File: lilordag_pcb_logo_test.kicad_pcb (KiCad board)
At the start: 2 copper layers, 98.1 x 100 mm, 178 parts, among them J1 USB4105-GF-A, J2 826629-7, J3 826629-7, Q1 BC846, Q2 BC846, Q3 MMBT3906, Q4 MMBT3906, Q5 BC846, Q6 BC846, Q7 SSM3J56MFV, Q8 SSM3J56MFV, SW1 PCM12SMTR, SW2 PCM12SMTR, SW3 SW_MEC_5G, SW4 PCM12SMTR, SW5 SW_MEC_5G, SW6 SW_MEC_5G, SW7 SW_MEC_5G, U1 ESP32-C3-MINI-1-N4, U2 WS2812B-B, U3 WS2812B-B, U4 WS2812B-B, U5 WS2812B-B

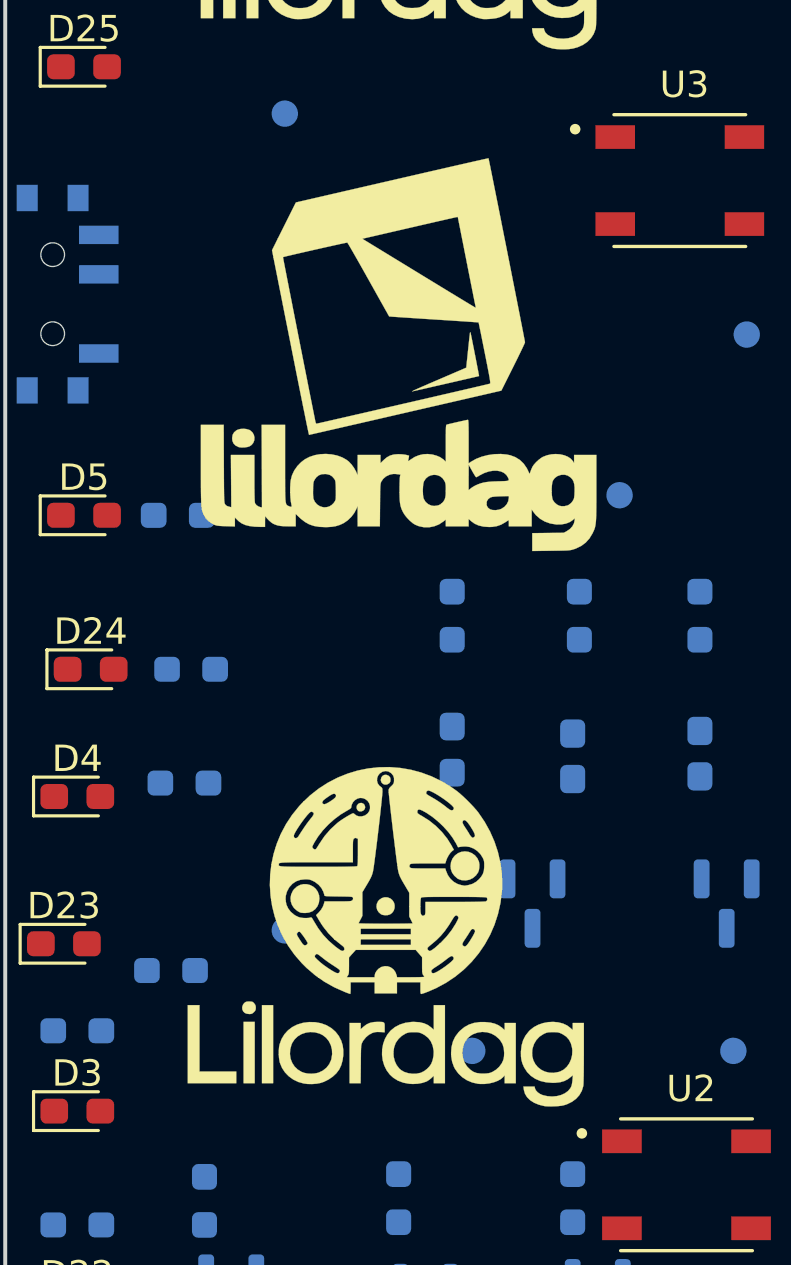
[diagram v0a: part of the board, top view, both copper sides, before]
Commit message: left lide logos locked
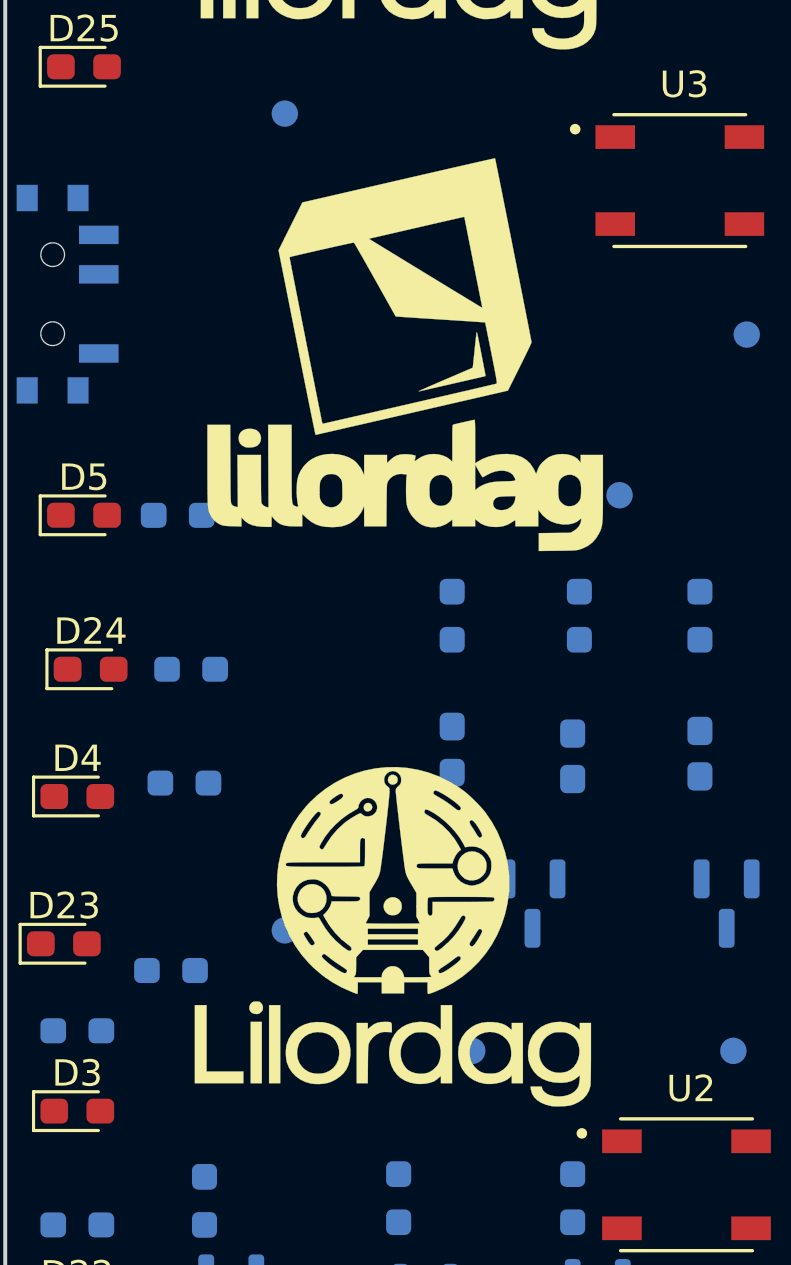
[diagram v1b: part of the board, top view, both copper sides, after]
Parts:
- moved Ref** 0.27 mm to (43.5, 87.4)
- moved Ref** 0.25 mm to (49.5, 73.2)
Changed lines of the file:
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@@
   )
   (footprint "pcb_logos:candy-simple-white" (layer "F.Cu")
-    (at 49.201917 73.168839)
+    (at 49.45 73.168839)
     (attr through_hole)
     (fp_text reference "Ref**" (at 0 0) (layer "F.SilkS") hide
@@
   )
   (footprint "pcb_logos:tower-complex-white" (layer "F.Cu")
-    (at 43.18 87.376)
+    (at 43.45 87.376)
     (attr through_hole)
     (fp_text reference "Ref**" (at 0 0) (layer "F.SilkS") hide
